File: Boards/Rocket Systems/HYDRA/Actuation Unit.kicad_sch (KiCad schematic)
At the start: 40 parts, among them Q10 2N7002H6327XTSA2, Q11 2N7002H6327XTSA2, U19 DRV103H, U20 DRV103H, U21 DRV103H, U22 DRV103H, U23 SQJA36EP-T1_GE3, U24 SQJA36EP-T1_GE3

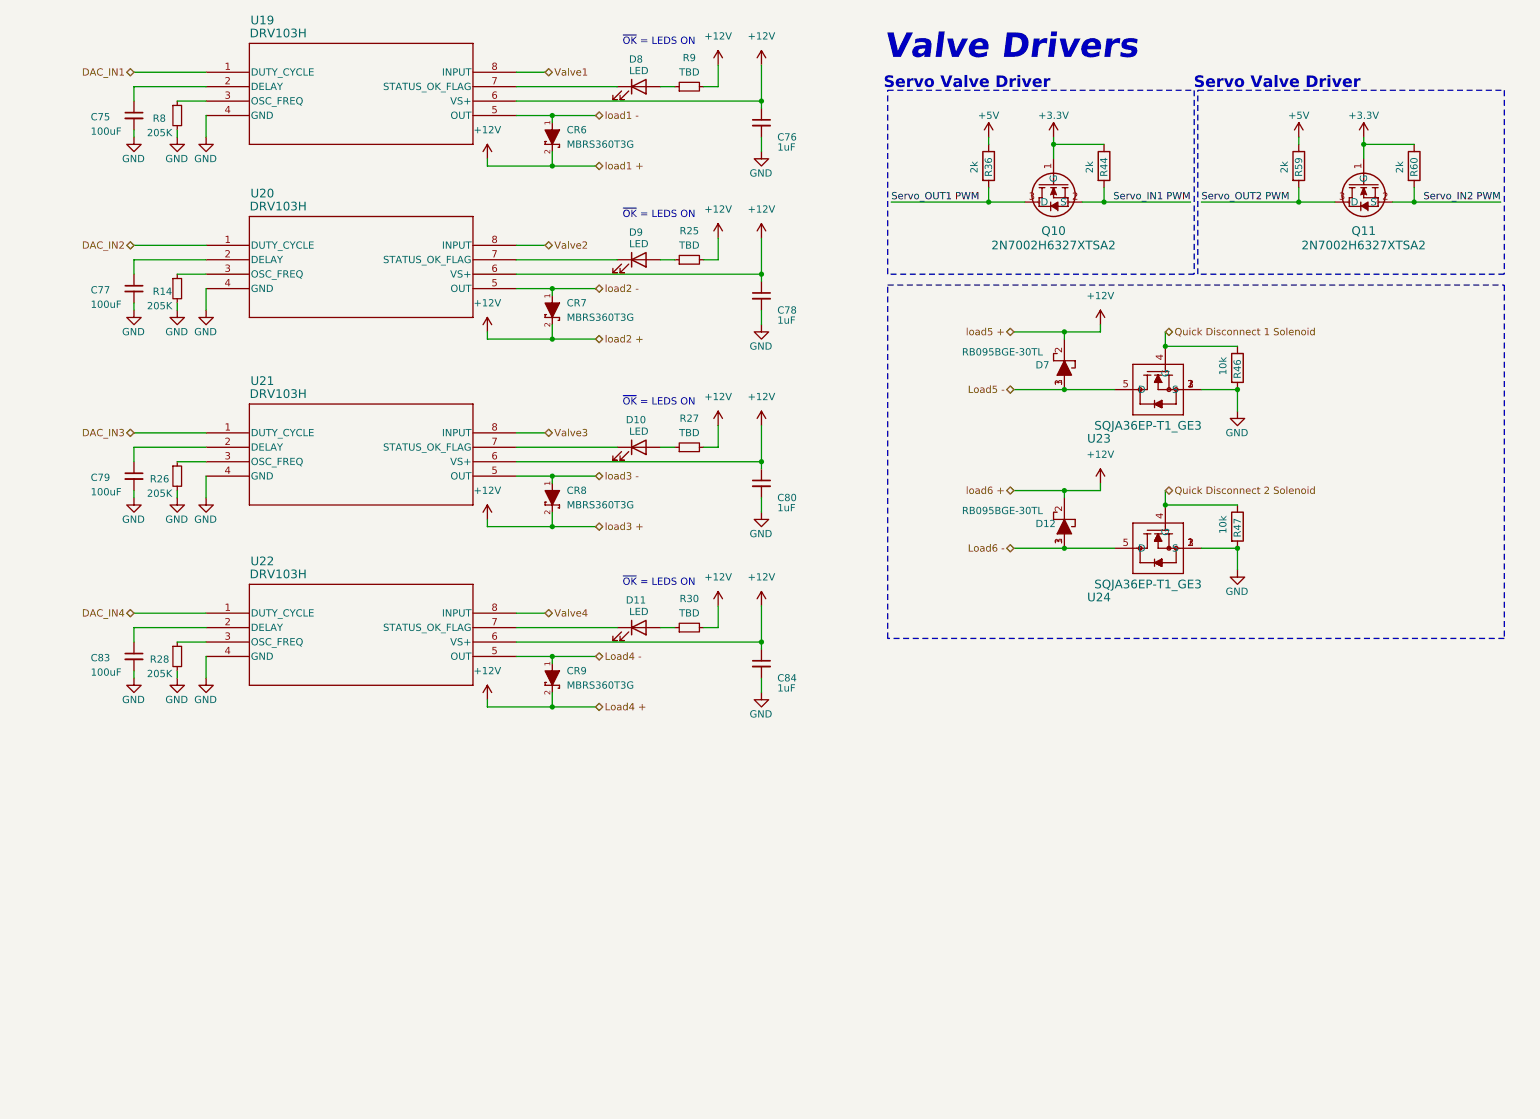
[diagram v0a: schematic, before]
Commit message: Full HYDRA UPDATE
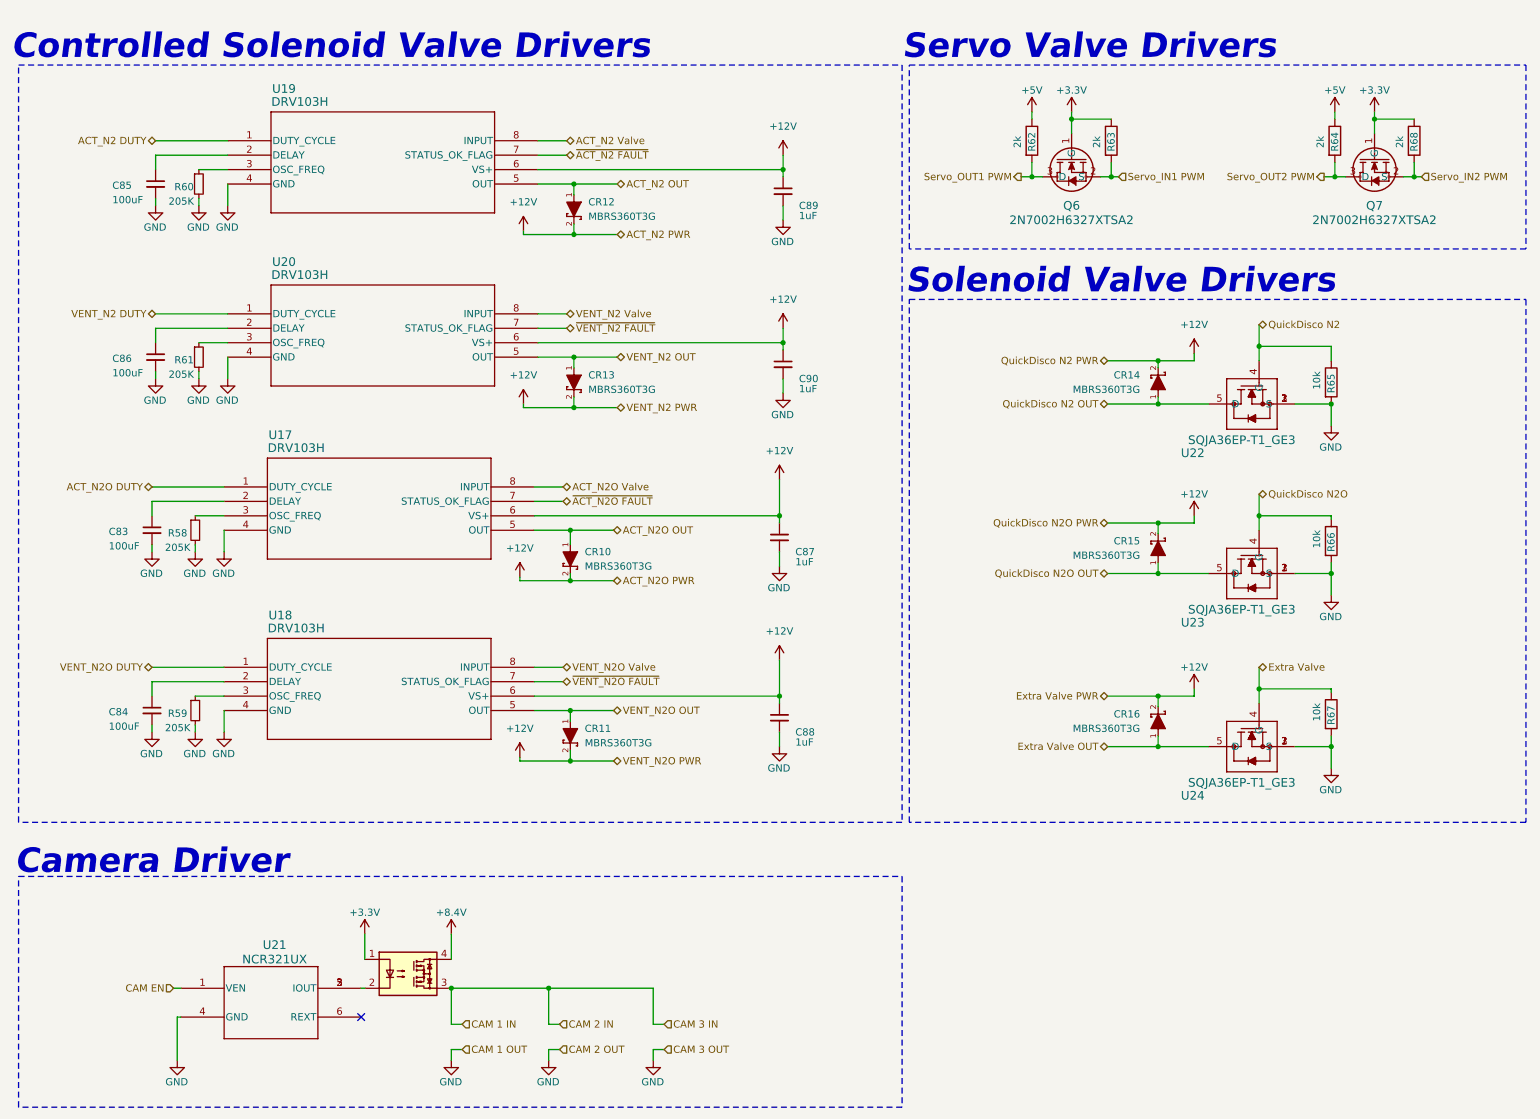
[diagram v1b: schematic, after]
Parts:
- removed D10, D11, D8, D9: LED, symbol Device:LED
- removed D12, D7: RB095BGE-30TL, RD3P175SNFRATL, symbol RB095BGE-30TL:RB095BGE-30TL
- removed Q11: 2N7002H6327XTSA2, NMOS_2N7002:PG-SOT23-3-5_INF_MIN, symbol NMOS_2N7002:2N7002H6327XTSA2
- removed R25, R27, R30, R9: TBD, symbol Device:R_Small
- removed R59, R60: 2k, Resistor-0402:RES_0402, symbol Device:R
- added CR14, CR15, CR16: MBRS360T3G, MBRS360T3G:DIODE_SMC_7P15X6P25_ONS-M, symbol MBRS360T3G:MBRS360T3G
- added K1: G3VM-31DR_TR05_, G3VM31DRTR05, symbol G3VM-31DR_TR05_:G3VM-31DR_TR05_
- added Q7: 2N7002H6327XTSA2, NMOS_2N7002:PG-SOT23-3-5_INF_MIN, symbol NMOS_2N7002:2N7002H6327XTSA2
- added R64, R68: 2k, Resistor-0402:RES_0402, symbol Device:R
- added R67: 10k, Resistor-0402:RES_0402, symbol Device:R
- added U21: NCR321UX, TSOP6_SOT457_NEX, symbol NCR321UX:NCR321UX
- added U24: SQJA36EP-T1_GE3, PowerPAK_SO-8L_3_VIS, symbol SQJA36EP-T1-GE3:SQJA36EP-T1_GE3
- renumbered C79 to C83, C83 to C84, C75 to C85, C77 to C86, C80 to C87, C84 to C88, C76 to C89, C78 to C90, CR8 to CR10, CR9 to CR11, CR6 to CR12, CR7 to CR13, Q10 to Q6, R26 to R58, R28 to R59, R8 to R60, R14 to R61, R36 to R62, R44 to R63, R46 to R65, R47 to R66, U21 to U17, U22 to U18, U23 to U22, U24 to U23
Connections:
- net +12V: now also CR14.2, CR15.2, CR16.2
- net +3.3V: now also K1.1, Q7.1 (G), R68.1
- net +5V: now also R64.1
- net GND: now also R67.2, U21.4 (GND), U24.1 (S), U24.2 (S), U24.3 (S)
- net Servo_IN2 PWM: now also Q7.2 (S), R68.2
- net Servo_OUT2 PWM: now also Q7.3 (D), R64.2
- net ~{ACT_N2O FAULT}: now reaches U17.7 (STATUS_OK_FLAG)
- net ~{VENT_N2 FAULT}: now reaches U20.7 (STATUS_OK_FLAG)
- net ~{VENT_N2O FAULT}: now reaches U18.7 (STATUS_OK_FLAG)
- net ~{ACT_N2 FAULT}: now reaches U19.7 (STATUS_OK_FLAG)
- net DAC_IN1 renamed ACT_N2 DUTY
- net DAC_IN2 renamed VENT_N2 DUTY
- net DAC_IN3 renamed ACT_N2O DUTY
- net DAC_IN4 renamed VENT_N2O DUTY
- net Load4 - renamed VENT_N2O OUT
- net Load5 - renamed QuickDisco N2 OUT
- net QuickDisco N2 OUT: now also CR14.1
- net Load6 - renamed QuickDisco N2O OUT
- net QuickDisco N2O OUT: now also CR15.1
- net Quick Disconnect 1 Solenoid renamed QuickDisco N2
- net Quick Disconnect 2 Solenoid renamed QuickDisco N2O
- net Valve1 renamed ACT_N2 Valve
- net Valve2 renamed VENT_N2 Valve
- net Valve3 renamed ACT_N2O Valve
- net Valve4 renamed VENT_N2O Valve
- net load1 - renamed ACT_N2 OUT
- net load2 - renamed VENT_N2 OUT
- net load3 - renamed ACT_N2O OUT
- new net: K1.2, U21.2 (IOUT), U21.3 (IOUT), U21.5 (IOUT)
- new net +8.4V: K1.4
- new net CAM 1 IN: K1.3
- new net CAM EN: U21.1 (VEN)
- new net Extra Valve: R67.1, U24.4 (G)
- new net Extra Valve OUT: CR16.1, U24.5 (D)
- no-connect marks 0 -> 1
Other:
- note added: "Camera Driver"
- note added: "Controlled Solenoid Valve Drivers"
- note added: "Servo Valve Drivers"
- note added: "Solenoid Valve Drivers"
- note removed: "Servo Valve Driver"
- note removed: "Valve Drivers"
- note removed: "~{OK} = LEDS ON"
- moved on the sheet: C83, C84, C85, C86, C87, C88, C89, C90, CR10, CR11, CR12, CR13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
